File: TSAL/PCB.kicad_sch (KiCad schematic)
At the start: 79 parts, among them J1 TE 770966-2, J2 JST B04B-XASK, J3 Conn_01x02, J4 Conn_01x02, Q1 IRLZ44N, Q2 MMBT3904, Q3 IRLZ44N, U1 TL431D, U2 LMV331, U3 UCC12040DVE, U4 LTV-817S, U5 LM555xN, U6 LF50_TO252, U7 MP174AGJ-Z

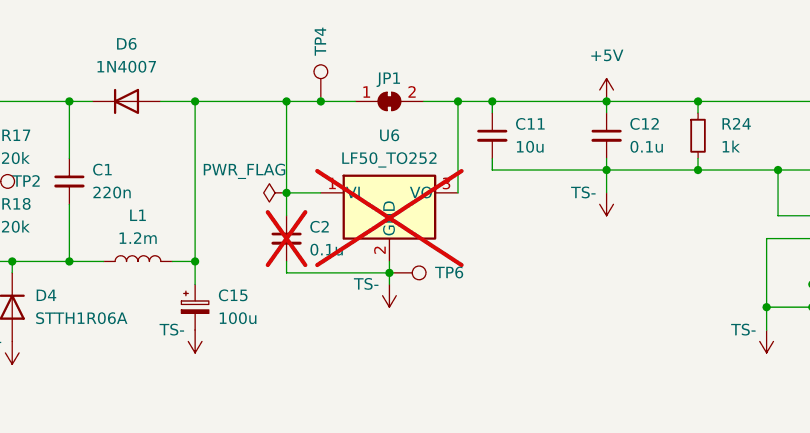
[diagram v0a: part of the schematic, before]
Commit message: JP1 Edit
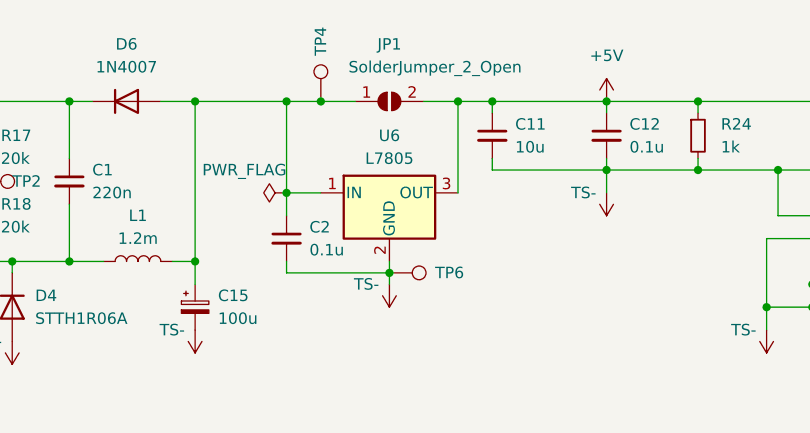
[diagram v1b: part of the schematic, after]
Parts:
- removed JP1: SolderJumper_2_Bridged, Jumper:SolderJumper-2_P1.3mm_Bridged_RoundedPad1.0x1.5mm, symbol Jumper:SolderJumper_2_Bridged
- added JP1: SolderJumper_2_Open, Jumper:SolderJumper-2_P1.3mm_Open_RoundedPad1.0x1.5mm, symbol Jumper:SolderJumper_2_Open
- C2: now fitted
- U6: value LF50_TO252 -> L7805; symbol Regulator_Linear:LF50_TO252 -> Regulator_Linear:L7805; now fitted
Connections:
- net +5V: now also JP1.2 (B)
- net at C15.1, C2.1, D6.2 (A)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: now also JP1.1 (A)
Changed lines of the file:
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@@
     )
   )
-  (symbol (lib_id "Regulator_Linear:LF50_TO252") (at 200.66 58.42 0) (unit 1)
-    (in_bom yes) (on_board yes) (dnp yes) (fields_autoplaced)
+  (symbol (lib_id "Regulator_Linear:L7805") (at 200.66 58.42 0) (unit 1)
+    (in_bom yes) (on_board yes) (dnp no) (fields_autoplaced)
     (property "Reference" "U6" (at 200.66 52.07 0)
       (effects (font (size 1.27 1.27)))
     )
-    (property "Value" "LF50_TO252" (at 200.66 54.61 0)
-      (effects (font (size 1.27 1.27)))
-    )
-    (property "Footprint" "Package_TO_SOT_SMD:TO-252-2" (at 200.66 52.705 0)
-      (effects (font (size 1.27 1.27) italic) hide)
-    )
-    (property "Datasheet" "http://www.st.com/content/ccc/resource/technical/document/datasheet/c4/0e/7e/2a/be/bc/4c/bd/CD00000546.pdf/files/CD00000546.pdf/jcr:content/translations/en.CD00000546.pdf" (at 200.66 59.69 0)
+    (property "Value" "L7805" (at 200.66 54.61 0)
+      (effects (font (size 1.27 1.27)))
+    )
+    (property "Footprint" "Package_TO_SOT_SMD:TO-252-2" (at 201.295 62.23 0)
+      (effects (font (size 1.27 1.27) italic) (justify left) hide)
+    )
+    (property "Datasheet" "http://www.st.com/content/ccc/resource/technical/document/datasheet/41/4f/b3/b0/12/d4/47/88/CD00000444.pdf/files/CD00000444.pdf/jcr:content/translations/en.CD00000444.pdf" (at 200.66 59.69 0)
       (effects (font (size 1.27 1.27)) hide)
     )
@@
     )
   )
+  (symbol (lib_id "Jumper:SolderJumper_2_Open") (at 200.66 48.26 0) (unit 1)
+    (in_bom yes) (on_board yes) (dnp no)
+    (property "Reference" "JP1" (at 200.66 41.91 0)
+      (effects (font (size 1.27 1.27)))
+    )
+    (property "Value" "SolderJumper_2_Open" (at 205.74 44.45 0)
+      (effects (font (size 1.27 1.27)))
+    )
+    (property "Footprint" "Jumper:SolderJumper-2_P1.3mm_Open_RoundedPad1.0x1.5mm" (at 200.66 48.26 0)
+      (effects (font (size 1.27 1.27)) hide)
+    )
+    (property "Datasheet" "~" (at 200.66 48.26 0)
+      (effects (font (size 1.27 1.27)) hide)
+    )
+    (pin "1")
+    (pin "2")
+    (instances
+      (project "PCB"
+        (path "/68f34db6-b185-48e2-8817-fb07f7d1240e"
+          (reference "JP1") (unit 1)
+        )
+      )
+    )
+  )
   (symbol (lib_id "Device:C_Small") (at 312.42 52.07 0) (unit 1)
     (in_bom yes) (on_board yes) (dnp no) (fields_autoplaced)
@@
   )
   (symbol (lib_id "Device:C_Small") (at 189.23 63.5 0) (unit 1)
-    (in_bom yes) (on_board yes) (dnp yes) (fields_autoplaced)
+    (in_bom yes) (on_board yes) (dnp no) (fields_autoplaced)
     (property "Reference" "C2" (at 191.77 62.2363 0)
       (effects (font (size 1.27 1.27)) (justify left))
@@
         )
       )
-    )
-  )
-  (symbol (lib_id "Jumper:SolderJumper_2_Bridged") (at 200.66 48.26 0) (unit 1)
-    (in_bom yes) (on_board yes) (dnp no)
-    (property "Reference" "JP1" (at 200.66 45.72 0)
-      (effects (font (size 1.27 1.27)))
-    )
-    (property "Value" "SolderJumper_2_Bridged" (at 200.66 44.45 0)
-      (effects (font (size 1.27 1.27)) hide)
-    )
-    (property "Footprint" "Jumper:SolderJumper-2_P1.3mm_Bridged_RoundedPad1.0x1.5mm" (at 200.66 48.26 0)
-      (effects (font (size 1.27 1.27)) hide)
-    )
-    (property "Datasheet" "~" (at 200.66 48.26 0)
-      (effects (font (size 1.27 1.27)) hide)
-    )
-    (pin "1")
-    (pin "2")
-    (instances
-      (project "PCB"
-        (path "/68f34db6-b185-48e2-8817-fb07f7d1240e"
-          (reference "JP1") (unit 1)
-        )
-      )
